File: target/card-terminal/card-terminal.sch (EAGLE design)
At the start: 33 parts, among them IC1 74S113D, Q1 16 MHz, Q2 BSS123, Q3 BSS123, Q4 BSS123, Q5 BSS123, Q6 BSS123, X2 5036-008-210-862

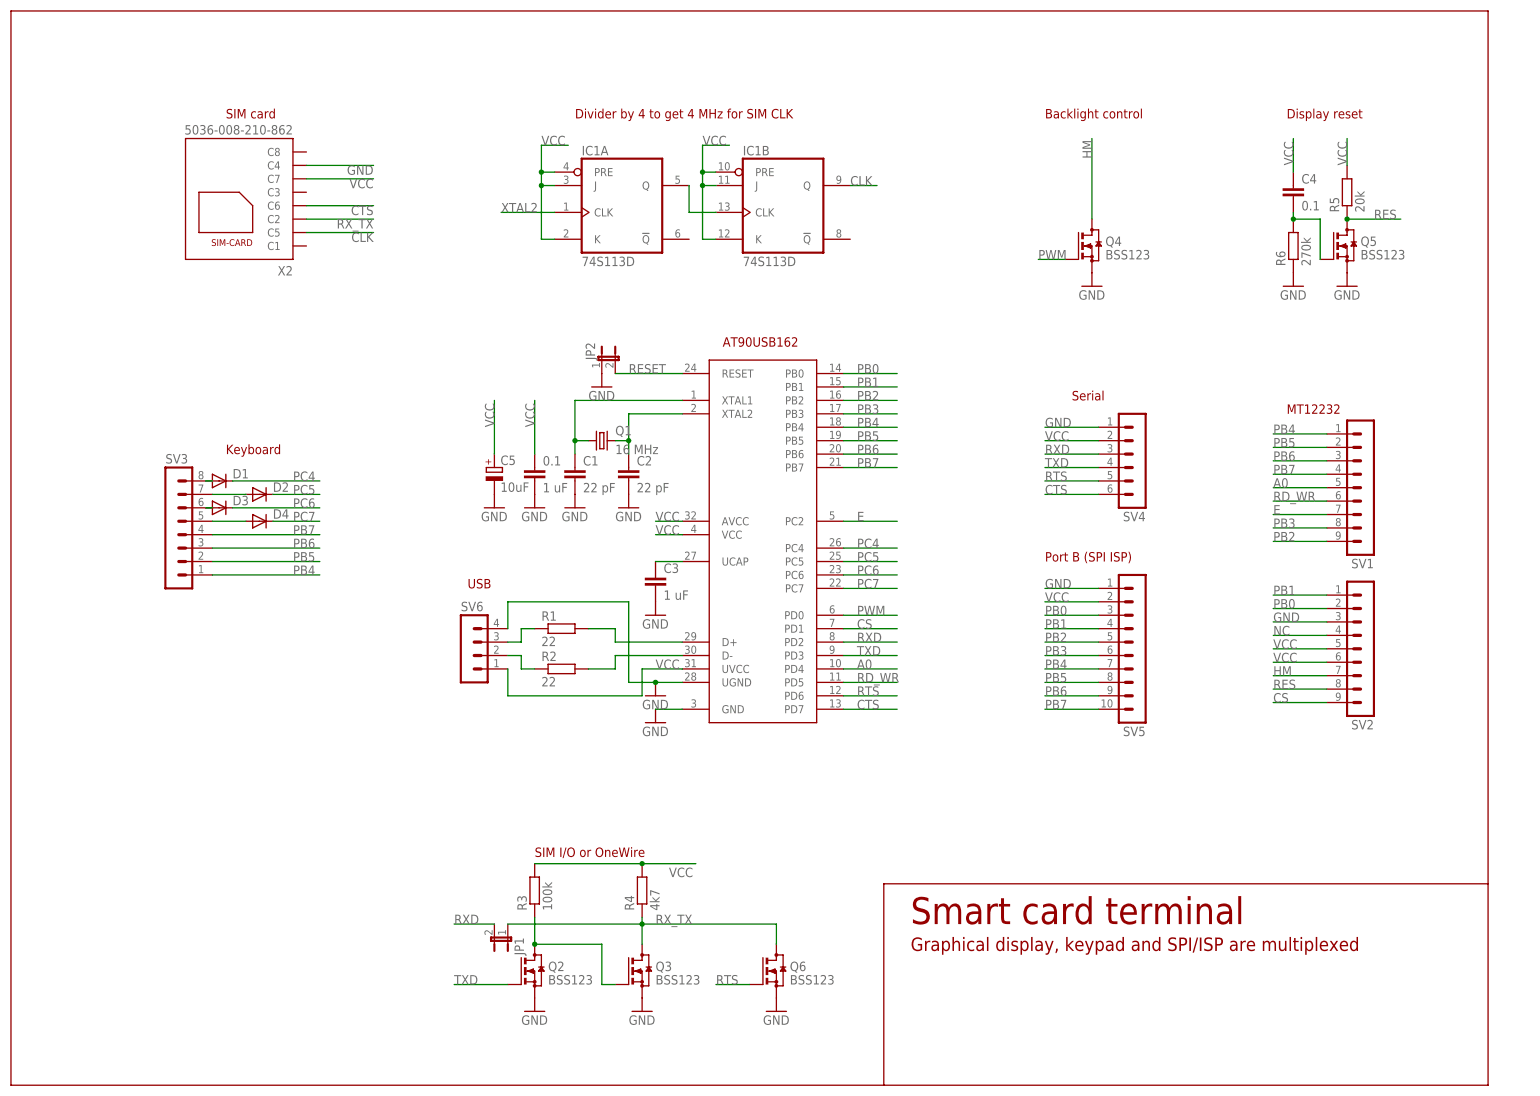
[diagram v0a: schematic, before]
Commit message: fixes for card-terminal hardware
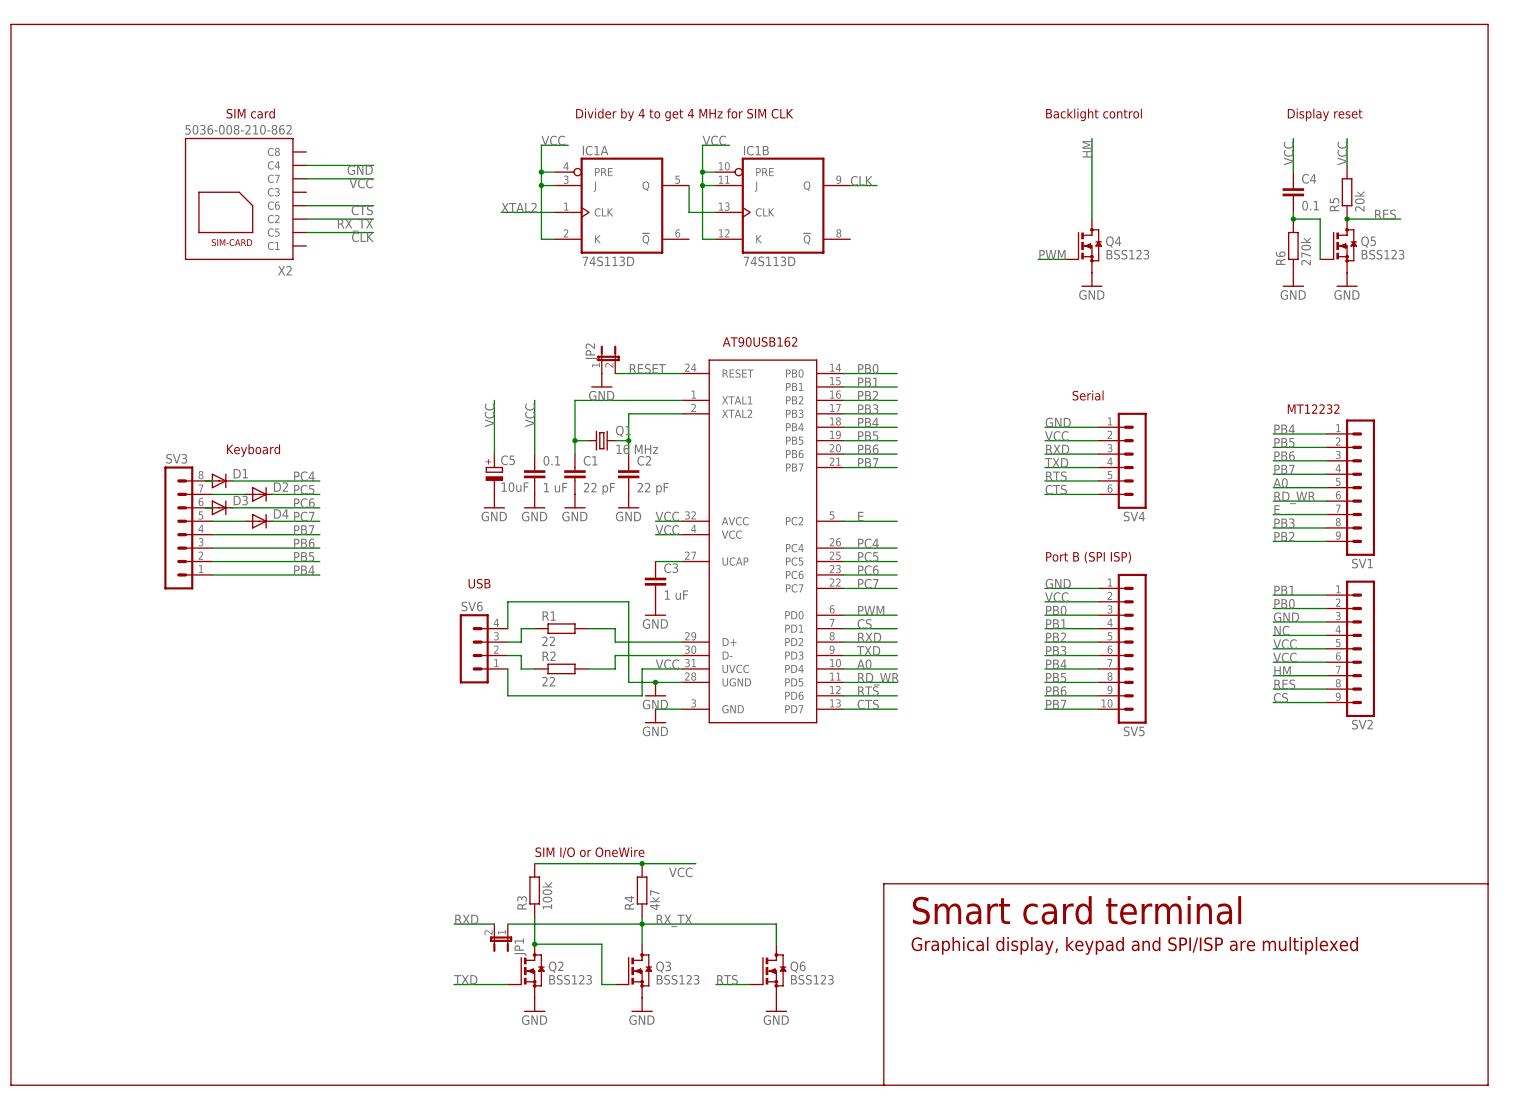
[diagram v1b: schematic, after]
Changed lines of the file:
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@@
 <setting verticaltext="up"/>
 </settings>
-<grid distance="0.1" unitdist="inch" unit="inch" style="lines" multiple="1" display="no" altdistance="0.01" altunitdist="inch" altunit="inch"/>
+<grid distance="0.1" unitdist="inch" unit="inch" style="lines" multiple="1" display="yes" altdistance="0.01" altunitdist="inch" altunit="inch"/>
 <layers>
 <layer number="1" name="Top" color="4" fill="1" visible="no" active="no"/>
@@
 <wire x1="0" y1="0" x2="165.1" y2="0" width="0.1524" layer="94"/>
 <wire x1="165.1" y1="0" x2="279.4" y2="0" width="0.1524" layer="94"/>
-<wire x1="279.4" y1="0" x2="279.4" y2="203.2" width="0.1524" layer="94"/>
-<wire x1="279.4" y1="203.2" x2="0" y2="203.2" width="0.1524" layer="94"/>
-<wire x1="0" y1="203.2" x2="0" y2="0" width="0.1524" layer="94"/>
+<wire x1="279.4" y1="0" x2="279.4" y2="200.66" width="0.1524" layer="94"/>
+<wire x1="279.4" y1="200.66" x2="0" y2="200.66" width="0.1524" layer="94"/>
+<wire x1="0" y1="200.66" x2="0" y2="0" width="0.1524" layer="94"/>
 <wire x1="279.4" y1="38.1" x2="165.1" y2="38.1" width="0.1524" layer="94"/>
 <wire x1="165.1" y1="38.1" x2="165.1" y2="0" width="0.1524" layer="94"/>
